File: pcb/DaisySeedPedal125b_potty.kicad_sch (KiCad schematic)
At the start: 3 parts, among them J6 Conn_01x20_Socket, J7 Conn_01x20_Socket

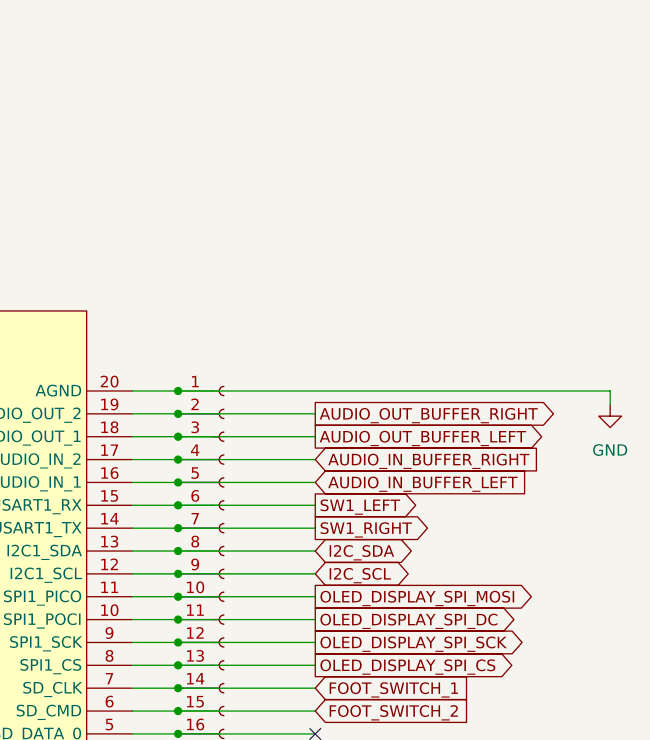
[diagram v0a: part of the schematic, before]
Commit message: Lots of updates to Schematic and pcb design
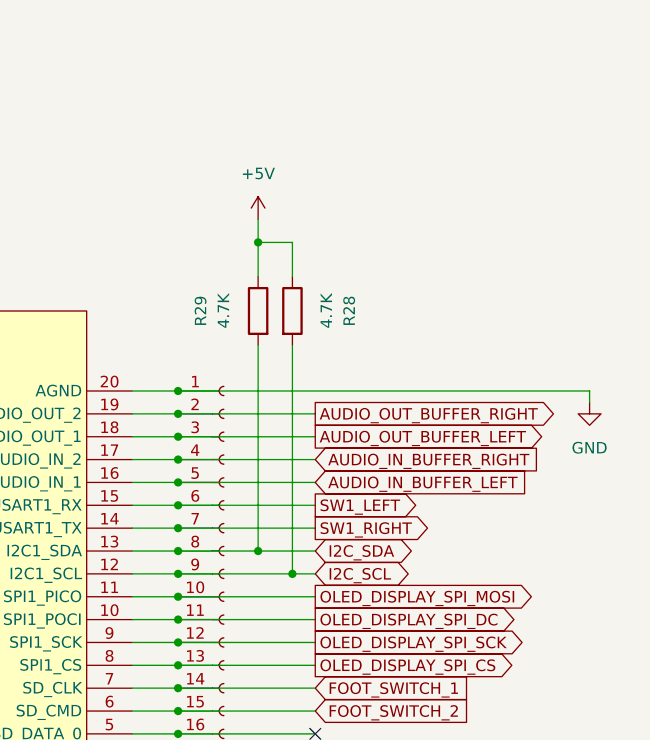
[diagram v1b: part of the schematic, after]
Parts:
- added R28, R29: 4.7K, Resistor_SMD:R_0805_2012Metric, symbol Device:R
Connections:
- net I2C_SCL: now also R28.2
- net I2C_SDA: now also R29.2
- new net +5V: R28.1, R29.1
